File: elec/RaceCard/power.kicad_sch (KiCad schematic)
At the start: 26 parts, among them J2 UJC-H-G-SMT-2-P6-TR, J3 530480210, Q1 DMP3125L-7, U3 MCP73812T-420I_OT, U4 TLV74033PDQNR, U5 AS11AH

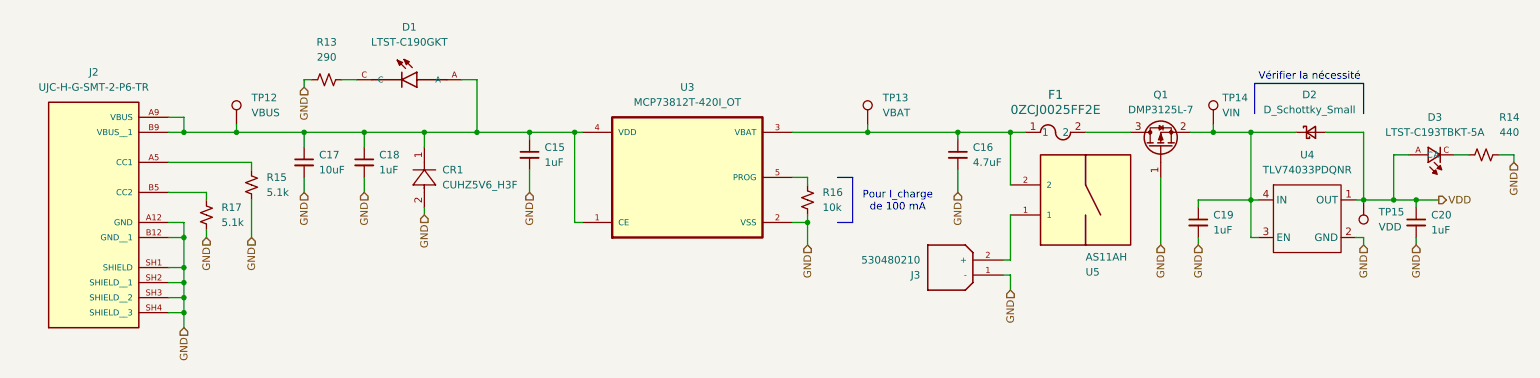
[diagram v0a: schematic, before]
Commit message: Power net update et cleanup sch
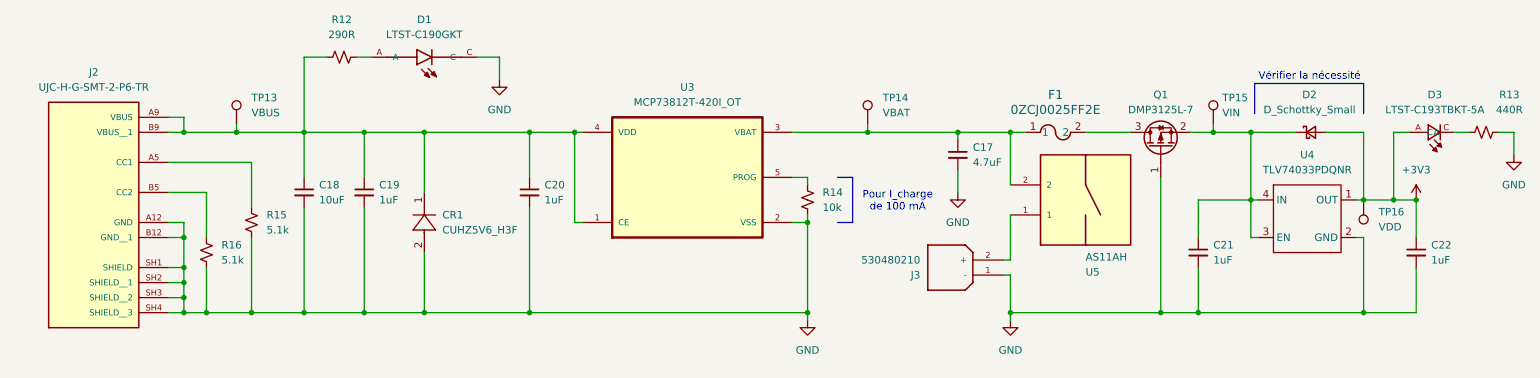
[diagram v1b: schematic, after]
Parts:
- R12: renamed from R13; value 290 -> 290R
- R13: renamed from R14; value 440 -> 440R
- renumbered C16 to C17, C17 to C18, C18 to C19, C15 to C20, C19 to C21, C20 to C22, R16 to R14, R17 to R16, TP12 to TP13, TP13 to TP14, TP14 to TP15, TP15 to TP16
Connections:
- net GND: now also D1.C; no longer R12.1
- net at C18.1, C19.1, C20.1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: now also R12.1; no longer D1.A
- net at R12.2: now also D1.A; no longer D1.C
- net VDD renamed +3V3
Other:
- moved on the sheet: C18, C19, C20, C21, C22, CR1, D1, D3, R12, R13, R15, R16
